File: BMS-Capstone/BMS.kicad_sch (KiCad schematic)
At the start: 0 parts

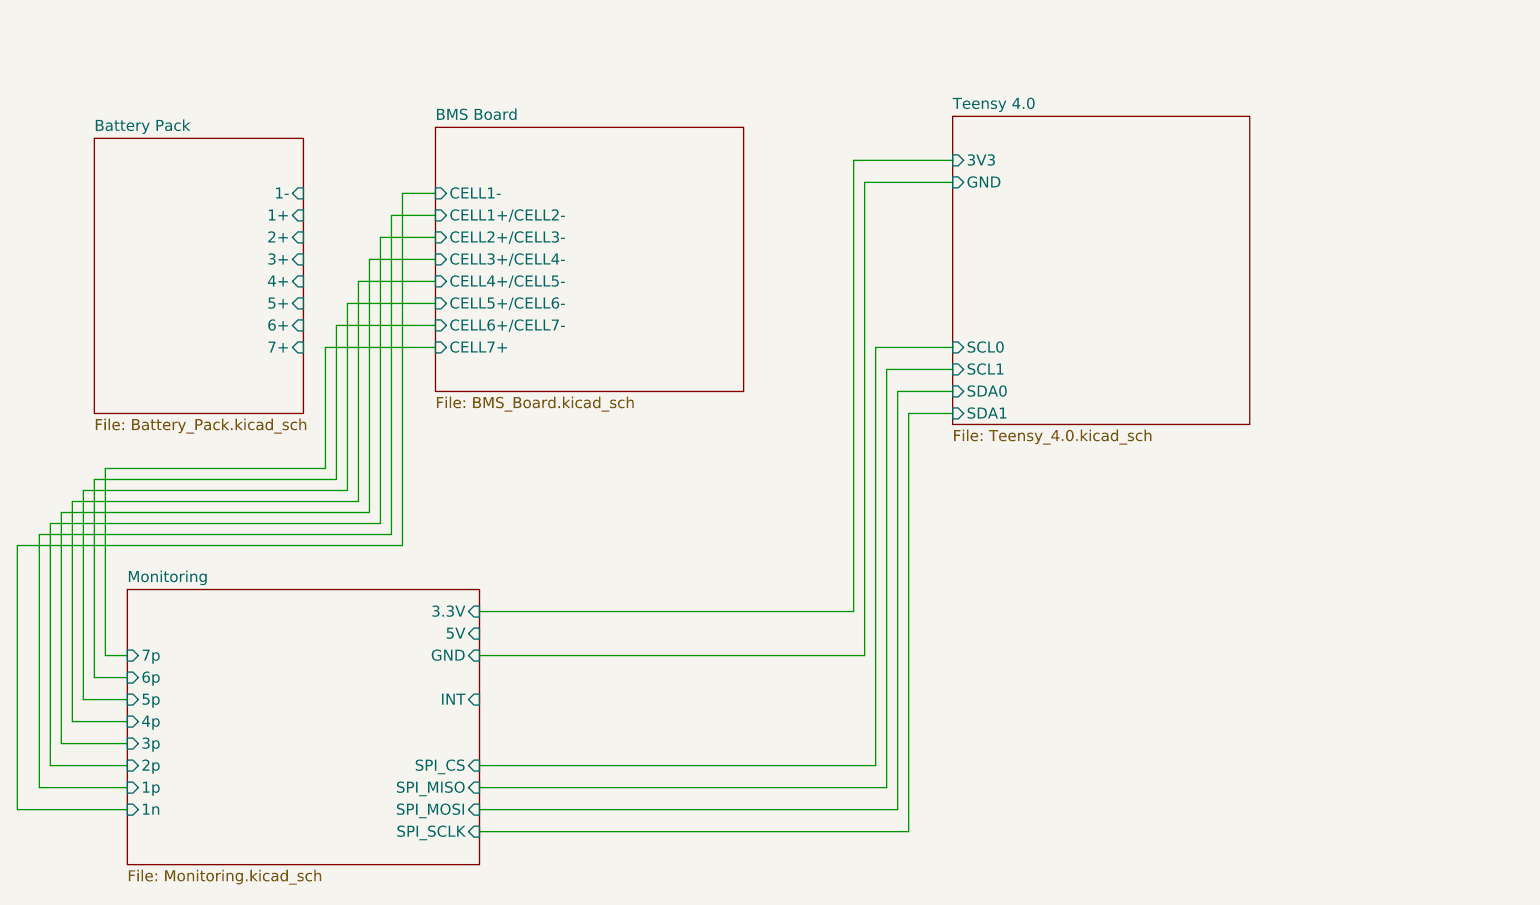
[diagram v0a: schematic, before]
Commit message: Final touches
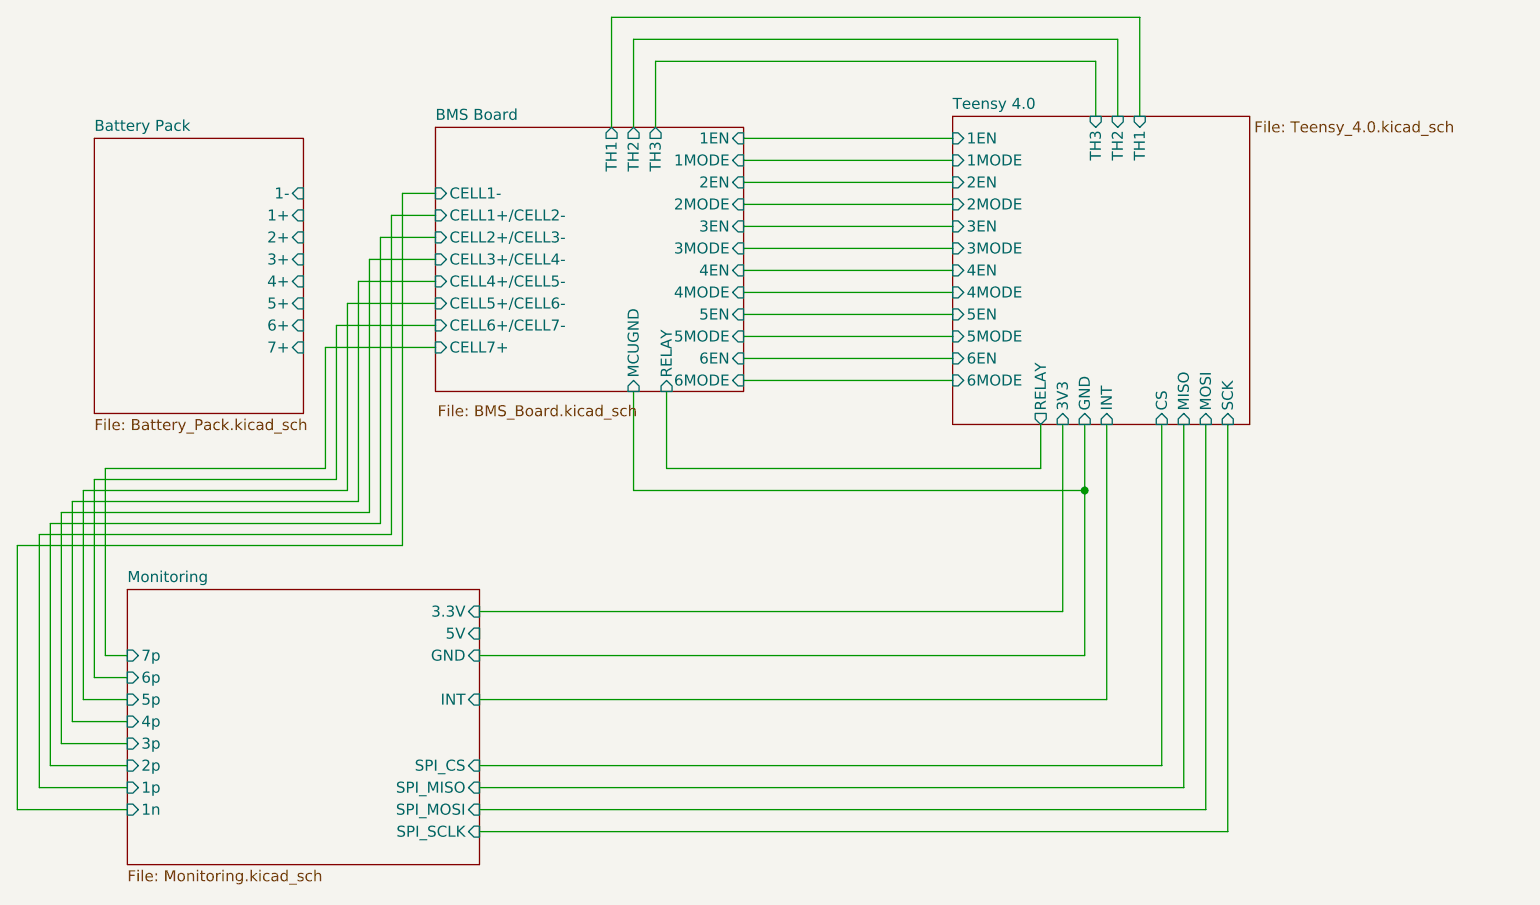
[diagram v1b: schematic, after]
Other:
- sheet BMS Board ports: added 1EN, 1MODE, 2EN, 2MODE, 3EN, 3MODE, 4EN, 4MODE, 5EN, 5MODE, 6EN, 6MODE, MCUGND, RELAY, TH1, TH2, TH3; removed none
- sheet Teensy 4.0 ports: added 1EN, 1MODE, 2EN, 2MODE, 3EN, 3MODE, 4EN, 4MODE, 5EN, 5MODE, 6EN, 6MODE, CS, INT, MISO, MOSI, RELAY, SCK, TH1, TH2, TH3; removed SCL0, SCL1, SDA0, SDA1
